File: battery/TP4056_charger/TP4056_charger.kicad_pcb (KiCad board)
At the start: 2 copper layers, 18 parts

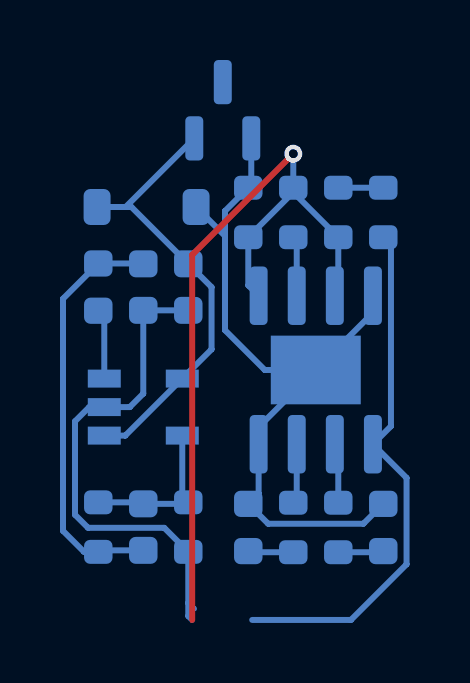
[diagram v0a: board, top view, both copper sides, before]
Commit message: update e-papert
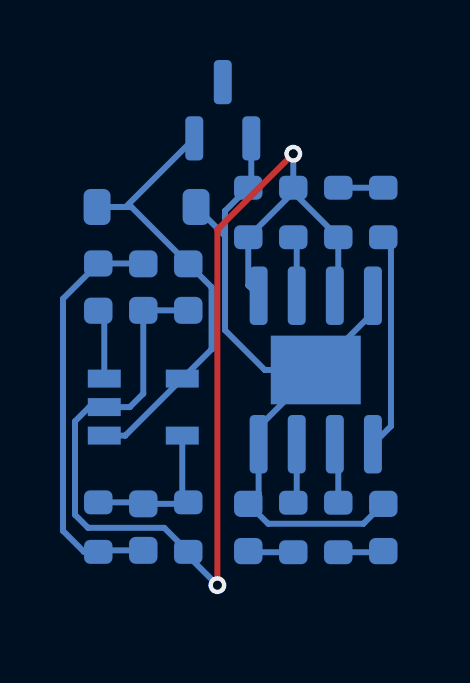
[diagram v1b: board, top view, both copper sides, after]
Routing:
- net VBAT: track 17.6 -> 7.25 mm
- net GND: track 43.5 -> 40.9 mm, vias 1 -> 2
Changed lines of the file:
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@@
 	)
 	(segment
-		(start -1.02 16.99)
-		(end -1.02 4.82)
+		(start 2.35 1.45)
+		(end -0.18 3.98)
 		(width 0.2)
 		(layer "F.Cu")
@@
 	)
 	(segment
-		(start -1.02 4.82)
-		(end 2.35 1.45)
+		(start -0.18 3.98)
+		(end -0.18 15.83)
 		(width 0.2)
 		(layer "F.Cu")
+		(net 1)
+	)
+	(via
+		(at -0.18 15.83)
+		(size 0.6)
+		(drill 0.3)
+		(layers "F.Cu" "B.Cu")
 		(net 1)
 	)
@@
 	)
 	(segment
-		(start -1.15 16.86)
-		(end -1.02 16.99)
-		(width 0.2)
-		(layer "B.Cu")
-		(net 1)
-	)
-	(segment
 		(start -4.452 9.895)
 		(end -3.95 9.895)
@@
 	)
 	(segment
+		(start -1.15 14.86)
+		(end -0.18 15.83)
+		(width 0.2)
+		(layer "B.Cu")
+		(net 1)
+	)
+	(segment
 		(start -2.65 6.67)
 		(end -2.65 9.445)
@@
 	)
 	(segment
-		(start -1.15 16.425)
-		(end -0.96 16.615)
-		(width 0.2)
-		(layer "B.Cu")
-		(net 1)
-	)
-	(segment
 		(start 2.35 2.7325)
 		(end 0.85 4.2325)
@@
 	)
 	(segment
+		(start -1.15 14.72)
+		(end -1.15 14.86)
+		(width 0.2)
+		(layer "B.Cu")
+		(net 1)
+	)
+	(segment
 		(start 0.85 4.2375)
 		(end 0.85 5.8375)
@@
 	)
 	(segment
-		(start -1.15 14.72)
-		(end -1.15 16.86)
-		(width 0.2)
-		(layer "B.Cu")
-		(net 1)
-	)
-	(segment
 		(start -4.926 10.369)
 		(end -4.452 9.895)
@@
 	)
 	(segment
-		(start 6.126 15.1351)
-		(end 6.126 12.2535)
-		(width 0.2)
-		(layer "B.Cu")
-		(net 13)
-	)
-	(segment
 		(start 5.35 4.2325)
 		(end 5.606 4.4885)
@@
 		(width 0.2)
 		(layer "B.Cu")
-		(net 13)
-	)
-	(segment
-		(start 6.126 12.2535)
-		(end 5.005 11.1325)
-		(width 0.2)
-		(layer "B.Cu")
-		(net 13)
-	)
-	(segment
-		(start 4.2711 16.99)
-		(end 6.126 15.1351)
-		(width 0.2)
-		(layer "B.Cu")
-		(net 13)
-	)
-	(segment
-		(start 0.98 16.99)
-		(end 4.2711 16.99)
-		(width 0.2)
-		(layer "B.Cu")
